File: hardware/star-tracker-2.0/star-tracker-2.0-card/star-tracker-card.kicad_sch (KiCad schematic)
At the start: 8 parts, among them J1 SM14B-SHLS-TF, J101 3-1734592-64-1734592-0, J4 TFM-120-01-L-D-RA, J7 GRPB041VWVN-RC

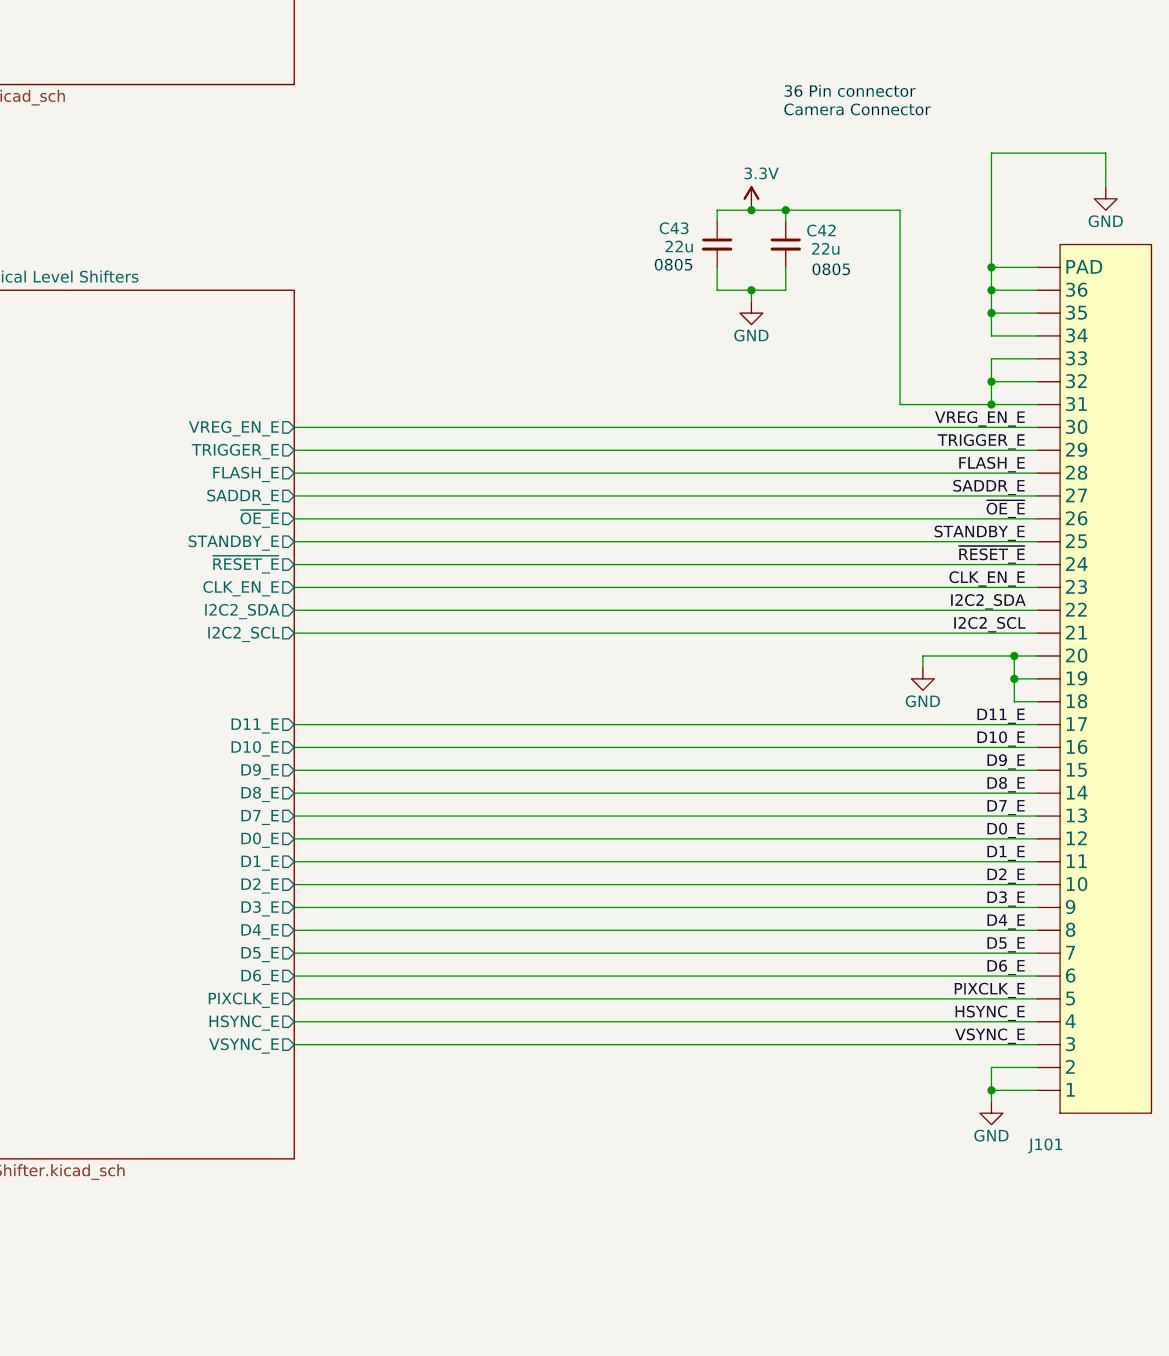
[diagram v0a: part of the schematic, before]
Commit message: Routine Push
Updated schematic and layout. about 60% done with routing.
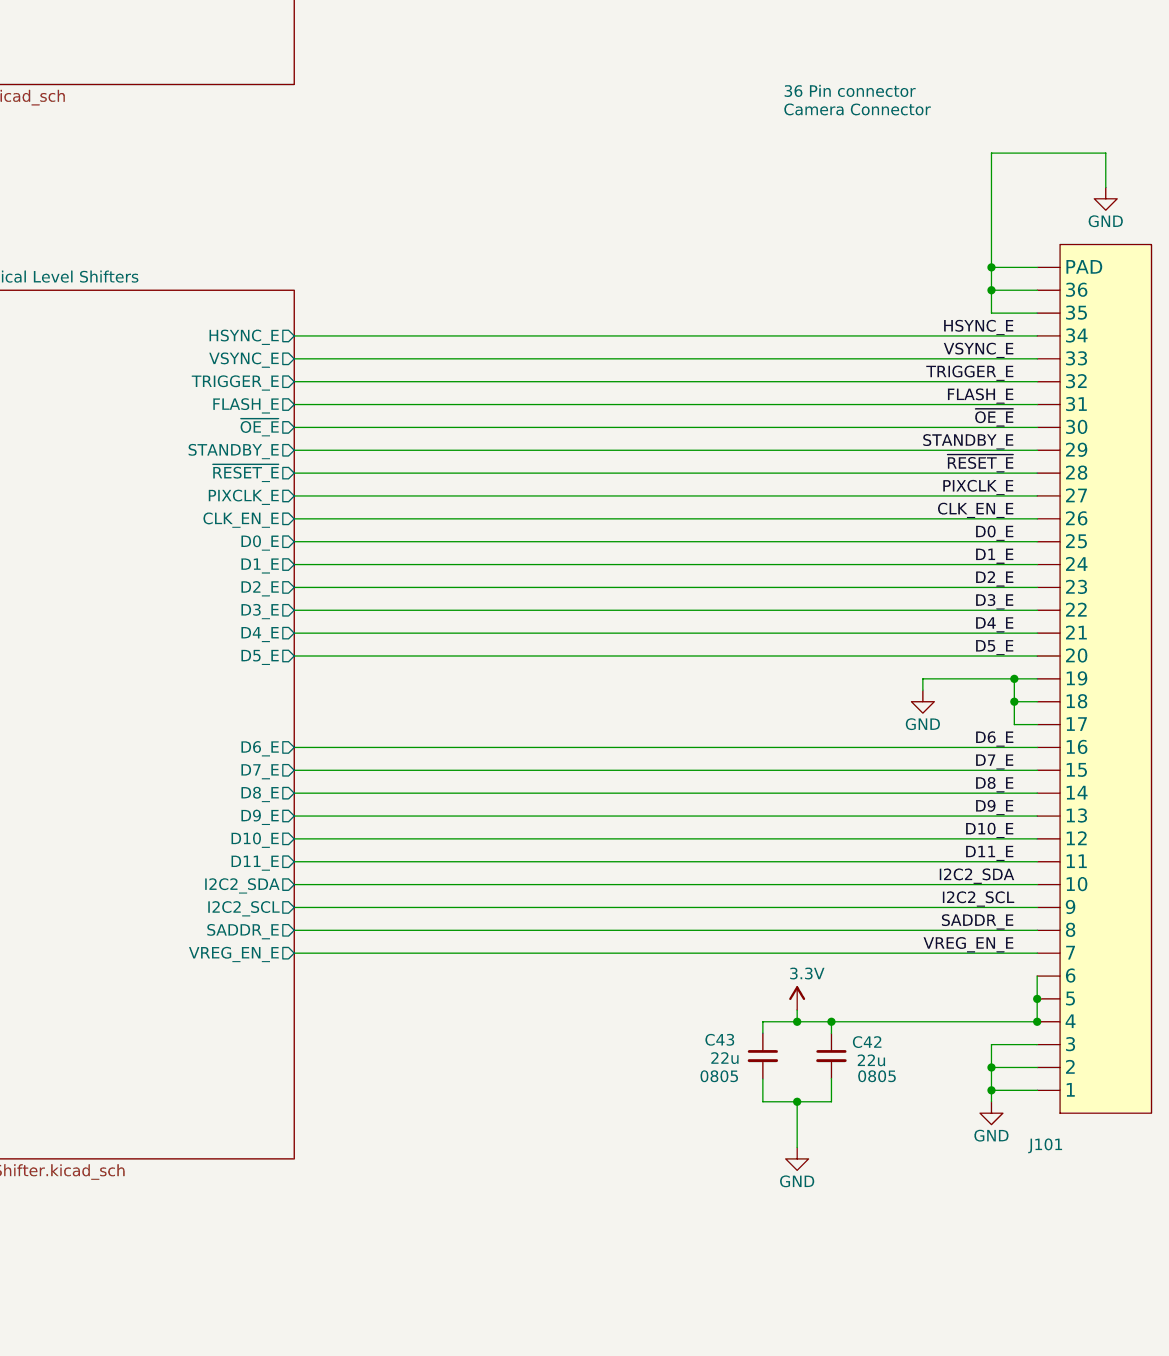
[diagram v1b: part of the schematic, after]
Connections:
- net 3.3V: now also J101.4, J101.5, J101.6; no longer J101.31, J101.32, J101.33
- net CLK_EN_E: now also J101.26; no longer J101.23
- net D0_E: now also J101.25; no longer J101.12
- net D10_E: now also J101.12; no longer J101.16
- net D11_E: now also J101.11; no longer J101.17
- net D1_E: now also J101.24; no longer J101.11
- net D2_E: now also J101.23; no longer J101.10
- net D3_E: now also J101.22; no longer J101.9
- net D4_E: now also J101.21; no longer J101.8
- net D5_E: now also J101.20; no longer J101.7
- net D6_E: now also J101.16; no longer J101.6
- net D7_E: now also J101.15; no longer J101.13
- net D9_E: now also J101.13; no longer J101.15
- net FLASH_E: now also J101.31; no longer J101.28
- net GND: now also J101.17, J101.3; no longer J101.20, J101.34
- net HSYNC_E: now also J101.34; no longer J101.4
- net I2C2_SCL: now also J101.9; no longer J101.21
- net I2C2_SDA: now also J101.10; no longer J101.22
- net PIXCLK_E: now also J101.27; no longer J101.5
- net SADDR_E: now also J101.8; no longer J101.27
- net STANDBY_E: now also J101.29; no longer J101.25
- net TRIGGER_E: now also J101.32; no longer J101.29
- net VREG_EN_E: now also J101.7; no longer J101.30
- net VSYNC_E: now also J101.33; no longer J101.3
- net ~{OE_E}: now also J101.30; no longer J101.26
- net ~{RESET_E}: now also J101.28; no longer J101.24
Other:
- moved on the sheet: C42, C43
